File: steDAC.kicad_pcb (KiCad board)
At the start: 2 copper layers, 100 x 80 mm, 153 parts, among them IC10 ADP7182ACPZN-R7, IC11 ADP150AUJZ-3.3-R7, IC2 ES9038Q2M, IC3 ATSAMS70N20A-AN, IC4 ADP150AUJZ-3.3-R7, IC5 ADP150AUJZ-3.3-R7, IC6 ADP150AUJZ-3.3-R7, IC7 ADP150AUJZ-3.3-R7, IC8 LT1026CS8#PBF, IC9 ADP7118ARDZ, J2 USB4105-GF-A, J3 Conn_02x05_Odd_Even, J5 Conn_01x02, J6 Conn_01x04, J7 STX-3120-5B-284C, U2 OPA1612-Q1, U3 OPA1612-Q1, U4 OPA1622, Y2 SiT8209AI-21-33S-100.000000X, Y3 12MHz

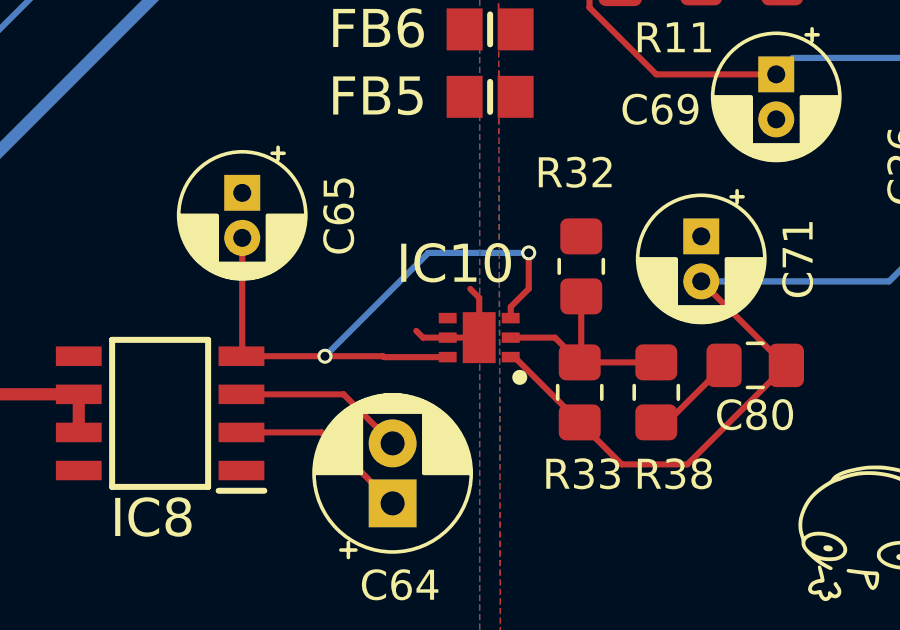
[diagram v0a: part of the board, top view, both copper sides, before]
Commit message: Trace edits
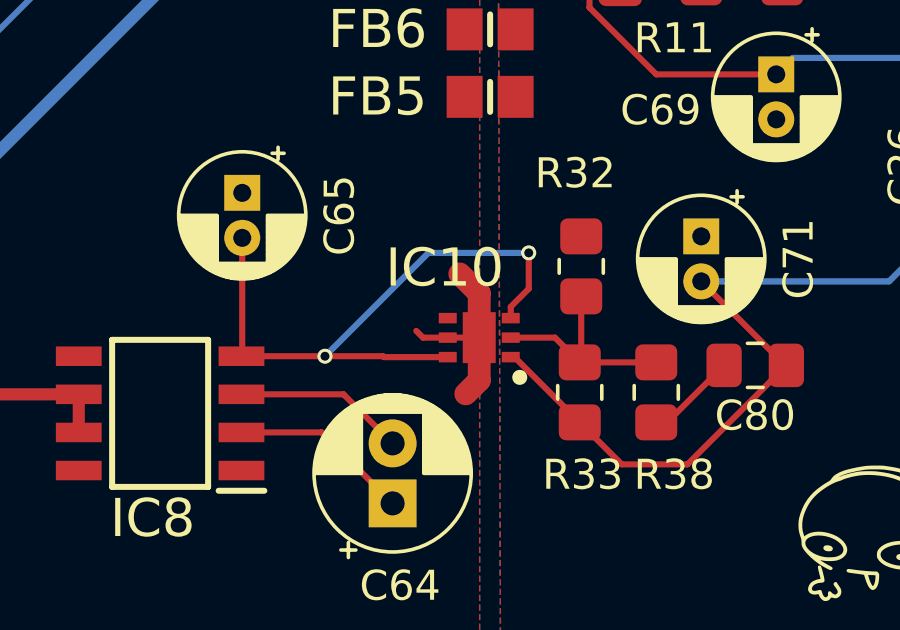
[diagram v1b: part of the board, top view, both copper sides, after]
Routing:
- net GND: track 28.0 -> 30.7 mm
